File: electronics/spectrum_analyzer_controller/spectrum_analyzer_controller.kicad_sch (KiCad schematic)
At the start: 45 parts, among them J1 AudioJack3, J2 Conn_02x03_Odd_Even, J3 Barrel_Jack_Switch, J4 Conn_01x10_Socket, J5 Conn_01x14_Socket, SW1 SW_SPDT, U1 MSGEQ7, U2 MSGEQ7, U3 ATtiny84-20P, U4 74HC595, U5 74HC595, U6 74HC595, U7 ULN2003, U8 ULN2003

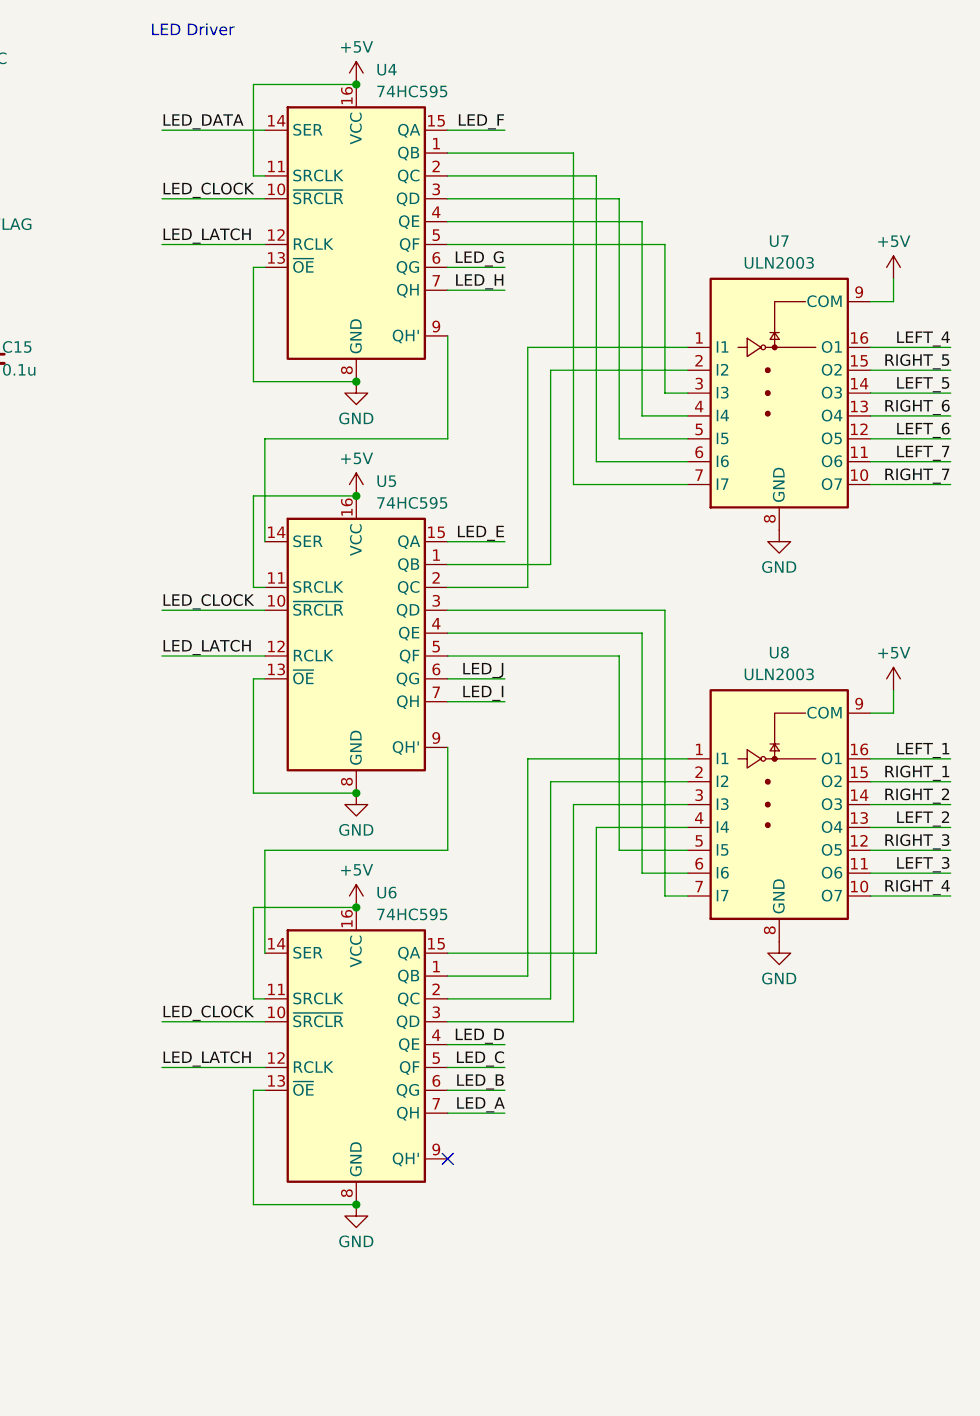
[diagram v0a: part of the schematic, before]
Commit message: chore: remove files
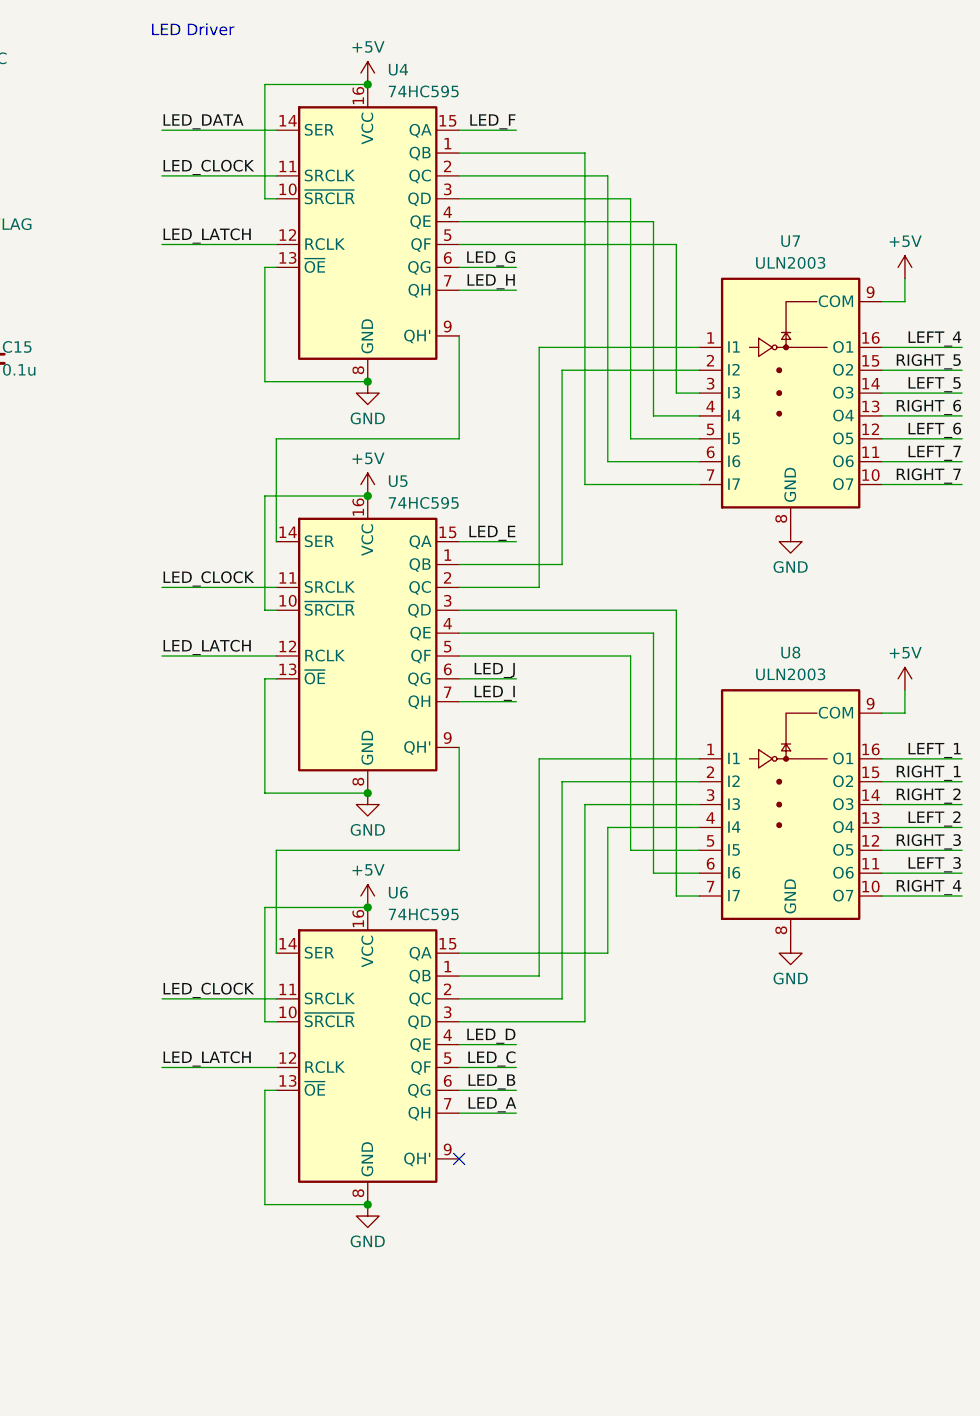
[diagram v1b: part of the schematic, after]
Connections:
- net +5V: now also U4.10 (~{SRCLR}), U5.10 (~{SRCLR}), U6.10 (~{SRCLR}); no longer U4.11 (SRCLK), U5.11 (SRCLK), U6.11 (SRCLK)
- net LED_CLOCK: now also U4.11 (SRCLK), U5.11 (SRCLK), U6.11 (SRCLK); no longer U4.10 (~{SRCLR}), U5.10 (~{SRCLR}), U6.10 (~{SRCLR})
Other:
- moved on the sheet: U4, U5, U6, U7, U8
